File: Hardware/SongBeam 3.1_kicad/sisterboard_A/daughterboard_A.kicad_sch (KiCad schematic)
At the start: 59 parts, among them J1 RJ45, J2 Conn_01x04, U1 PCMD3180IRTWR, U10 LP5907MFX-1.8_NOPB, U2 IM66D132H, U3 IM66D132H, U4 IM66D132H, U5 IM66D132H, U6 IM66D132H, U7 IM66D132H, U8 IM66D132H, U9 IM66D132H

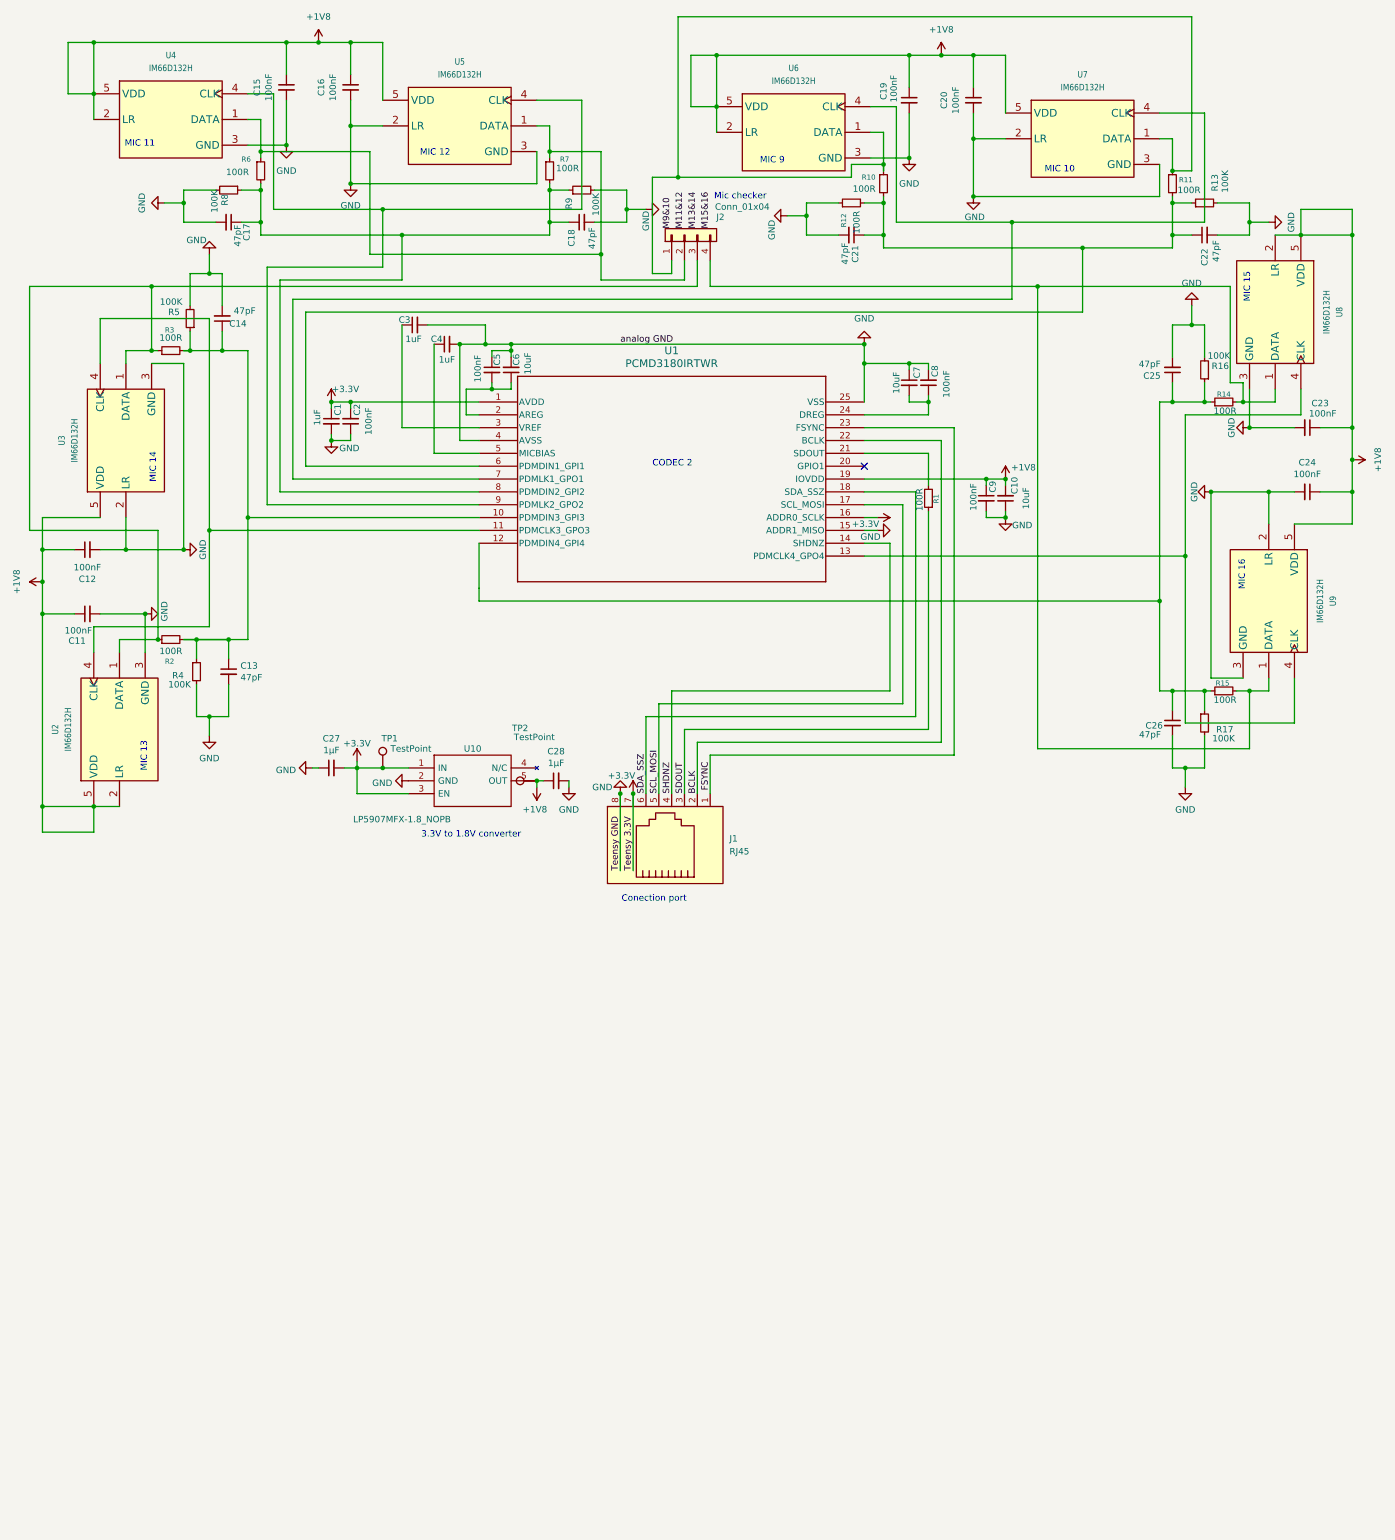
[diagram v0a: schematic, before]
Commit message: Layout updates
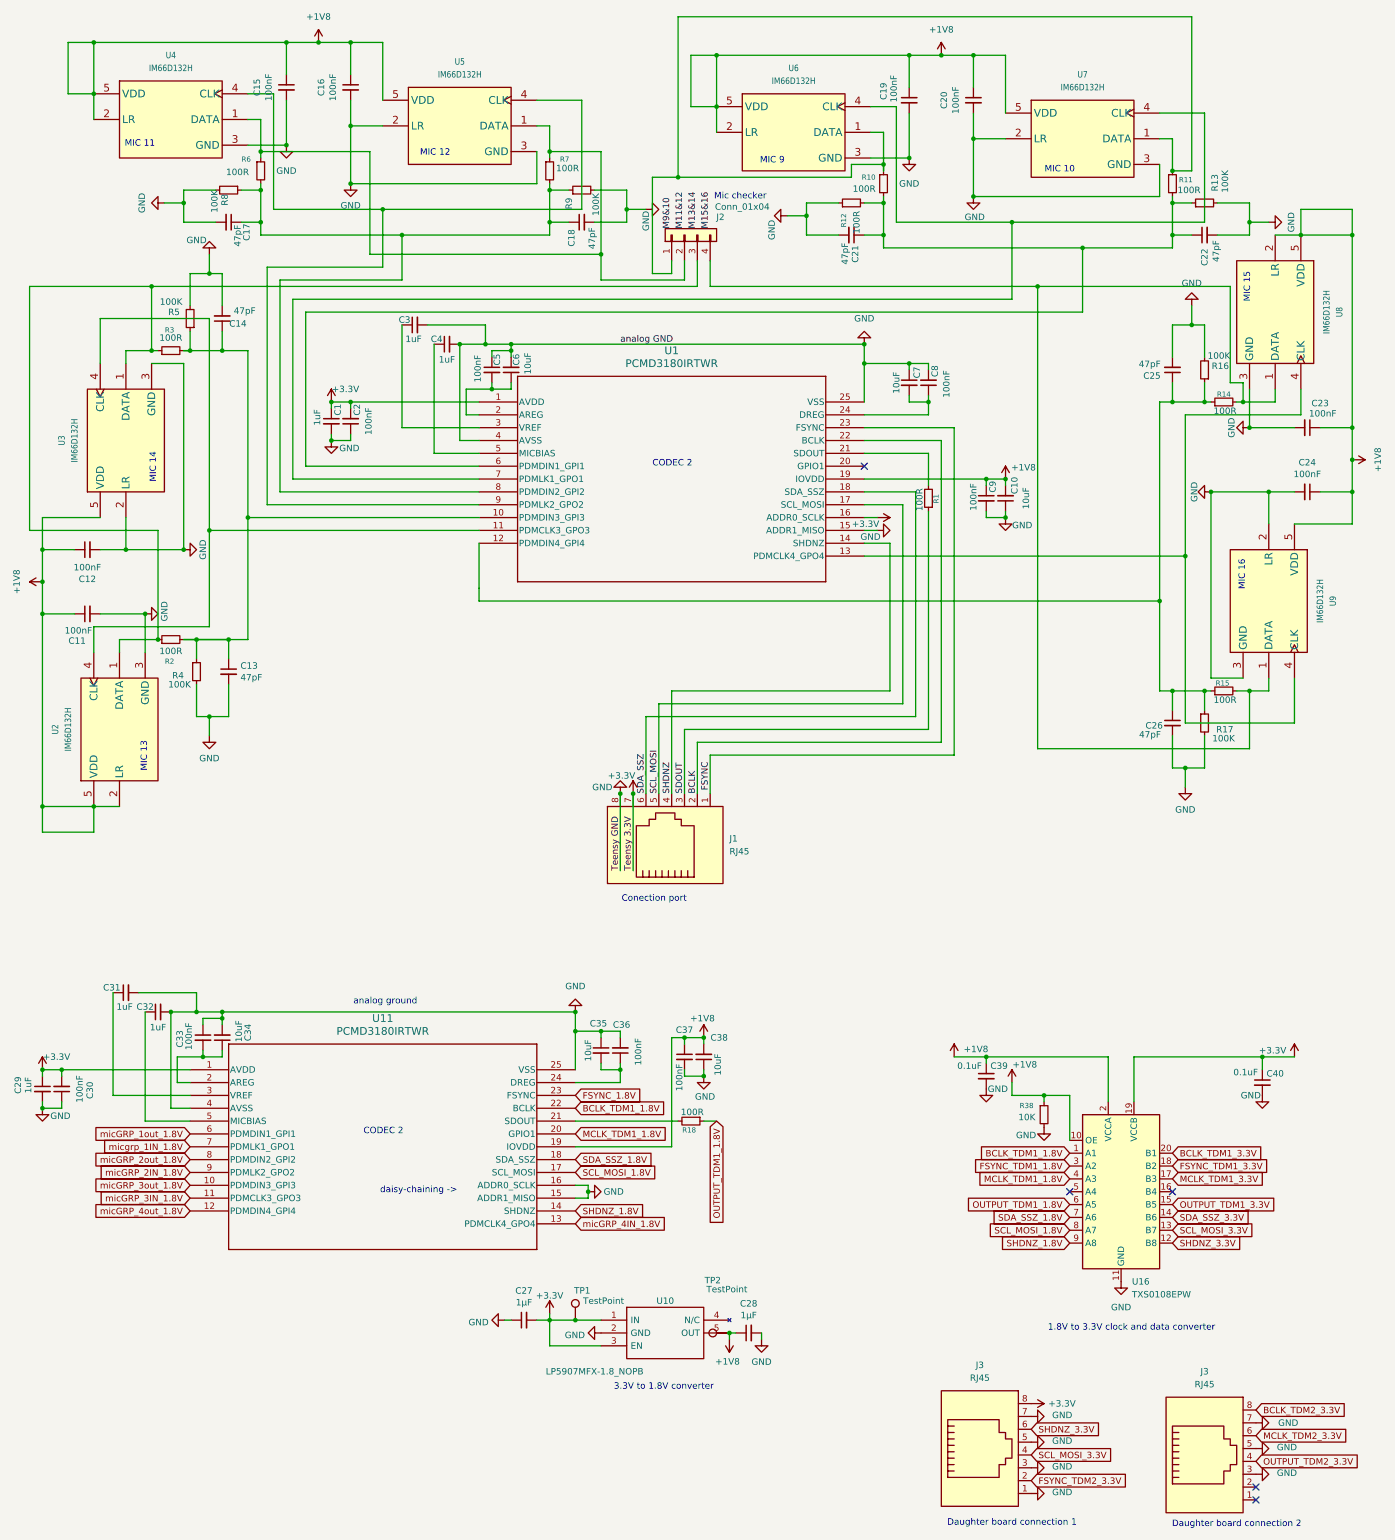
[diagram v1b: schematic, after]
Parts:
- added C29, C31, C32: 1uF, Capacitor_SMD:C_0805_2012Metric, symbol Device:C_Small
- added C30, C33, C36, C37: 100nF, Capacitor_SMD:C_0805_2012Metric, symbol Device:C_Small
- added C34, C35, C38: 10uF, Capacitor_SMD:C_0805_2012Metric, symbol Device:C_Small
- added C39, C40: 0.1uF, Capacitor_SMD:C_0805_2012Metric, symbol Device:C_Small
- added J3 (x2): RJ45, RJHSE-3380:CONN_RJHSE-3380_AMP, symbol Connector:RJ45
- added R18: 100R, Resistor_SMD:R_0805_2012Metric, symbol Device:R_Small
- added R38: 10K, Resistor_SMD:R_0805_2012Metric, symbol Device:R_Small
- added U11: PCMD3180IRTWR, PCMD3180IRTWR:PCMD3180IRTWR, symbol PCMD3180:PCMD3180IRTWR
- added U16: TXS0108EPW, Package_SO:TSSOP-20_4.4x6.5mm_P0.65mm, symbol Logic_LevelTranslator:TXS0108EPW
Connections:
- net +1V8: now also C37.1, C38.2, C39.1, R38.1, U11.19 (IOVDD), U16.10 (OE), U16.2 (VCCA)
- net +3.3V: now also C29.1, C30.2, C40.1, J3.8, U11.1 (AVDD), U16.19 (VCCB)
- net GND: now also C29.2, C30.1, C31.2, C32.2, C33.1, C34.2, C35.1, C36.2, C37.2, C38.1, C39.2, C40.2, J3.1, J3.3, J3.3, J3.5, J3.5, J3.7, J3.7, R38.2, U11.15 (ADDR1_MISO), U11.16 (ADDR0_SCLK), U11.25 (VSS), U11.4 (AVSS), U16.11 (GND)
- new net: C31.1, U11.3 (VREF)
- new net: C33.2, C34.1, U11.2 (AREG)
- new net: R18.2, U11.21 (SDOUT)
- new net: C35.2, C36.1, U11.24 (DREG)
- new net: C32.1, U11.5 (MICBIAS)
- new net BCLK_TDM1_1.8V: U11.22 (BCLK), U16.1 (A1)
- new net BCLK_TDM1_3.3V: U16.20 (B1)
- new net BCLK_TDM2_3.3V: J3.8
- new net FSYNC_1.8V: U11.23 (FSYNC)
- new net FSYNC_TDM1_1.8V: U16.3 (A2)
- new net FSYNC_TDM1_3.3V: U16.18 (B2)
- new net FSYNC_TDM2_3.3V: J3.2
- new net MCLK_TDM1_1.8V: U11.20 (GPIO1), U16.4 (A3)
- new net MCLK_TDM1_3.3V: U16.17 (B3)
- new net MCLK_TDM2_3.3V: J3.6
- new net OUTPUT_TDM1_1.8V: R18.1, U16.6 (A5)
- new net OUTPUT_TDM1_3.3V: U16.15 (B5)
- new net OUTPUT_TDM2_3.3V: J3.4
- new net SCL_MOSI_1.8V: U11.17 (SCL_MOSI), U16.8 (A7)
- new net SCL_MOSI_3.3V: J3.4, U16.13 (B7)
- new net SDA_SSZ_1.8V: U11.18 (SDA_SSZ), U16.7 (A6)
- new net SDA_SSZ_3.3V: U16.14 (B6)
- new net SHDNZ_1.8V: U11.14 (SHDNZ), U16.9 (A8)
- new net SHDNZ_3.3V: J3.6, U16.12 (B8)
- new net micGRP_1out_1.8V: U11.6 (PDMDIN1_GPI1)
- new net micGRP_2IN_1.8V: U11.9 (PDMLK2_GPO2)
- new net micGRP_2out_1.8V: U11.8 (PDMDIN2_GPI2)
- new net micGRP_3IN_1.8V: U11.11 (PDMCLK3_GPO3)
- new net micGRP_3out_1.8V: U11.10 (PDMDIN3_GPI3)
- new net micGRP_4IN_1.8V: U11.13 (PDMCLK4_GPO4)
- new net micGRP_4out_1.8V: U11.12 (PDMDIN4_GPI4)
- new net micgrp_1IN_1.8V: U11.7 (PDMLK1_GPO1)
- no-connect marks 1 -> 5
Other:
- note added: "1.8V to 3.3V clock and data converter"
- note added: "Daughter board connection 1"
- note added: "Daughter board connection 2"
- note added: "analog ground"
- note added: "daisy-chaining ->"
- moved on the sheet: C27, C28, TP1, TP2, U10
